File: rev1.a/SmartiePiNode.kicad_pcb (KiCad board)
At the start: 2 copper layers, 71.7 x 55 mm, 62 parts, among them CN1 USBMICROb, CN2 SWD, CN3 SX1238_TRX_HEADER, CN4 VIN, SW1 SW_PUSH, U1 ISL91127IR, U2 STM32L052_LQFP48, X1 abm10, X2 ABS25-32.768KHZ-6-T

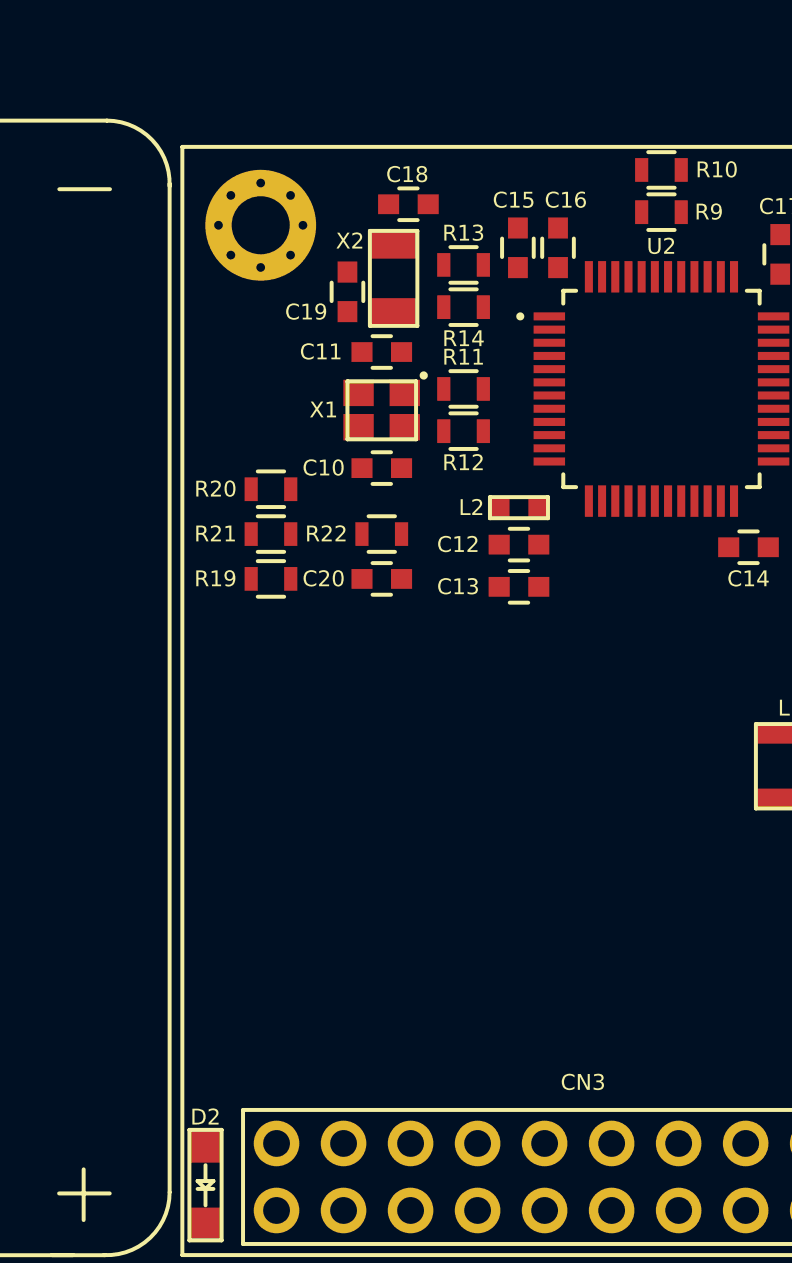
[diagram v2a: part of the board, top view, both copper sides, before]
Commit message: more layout
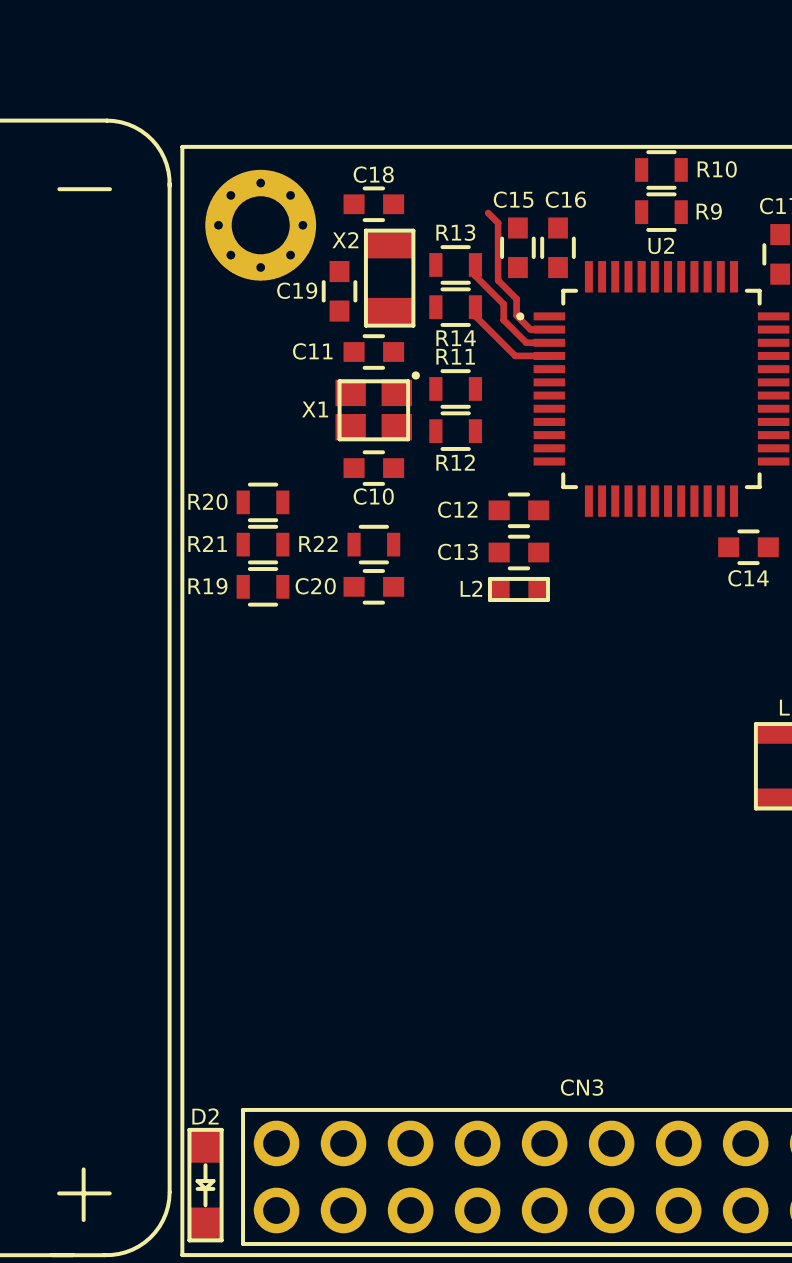
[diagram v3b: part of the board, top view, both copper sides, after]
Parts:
- moved L2 3.10 mm to (143.3, 124.8)
- moved C18 1.31 mm to (137.8, 110.2), turned to 0 degrees
- moved C12 1.30 mm to (143.3, 121.8)
- moved C13 1.30 mm to (143.3, 123.4)
- moved R20 0.58 mm to (133.6, 121.5)
- moved R21 0.50 mm to (133.6, 123.1)
- moved R22 0.50 mm to (137.8, 123.1)
- moved R19 0.42 mm to (133.6, 124.7)
- moved C20 0.42 mm to (137.8, 124.7)
- moved C19 0.30 mm to (136.5, 113.5)
- moved C10 0.30 mm to (137.8, 120.2)
- moved C11 0.30 mm to (137.8, 115.8)
- moved R11 0.30 mm to (140.9, 117.2)
- moved R12 0.30 mm to (140.9, 118.8), turned to 180 degrees
- moved R13 0.30 mm to (140.9, 112.5)
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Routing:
- net Net-(U2-Pad2): track 0.00 -> 5.80 mm
- net Net-(R13-Pad2): track 0.00 -> 4.62 mm
- net Net-(R14-Pad2): track 0.00 -> 3.77 mm
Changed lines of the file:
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@@
   (general
     (links 205)
-    (no_connects 141)
+    (no_connects 139)
     (area 98.984999 95.604999 170.825001 150.735001)
     (thickness 1.6)
     (drawings 12)
-    (tracks 1)
+    (tracks 15)
     (zones 0)
     (modules 62)
@@
   )
   (module Capacitors_SMD:C_0603 (layer F.Cu)
-    (at 138.1 120.2 180)
+    (at 137.8 120.2 180)
     (descr "Capacitor SMD 0603, reflow soldering, AVX (see smccp.pdf)")
     (tags "capacitor 0603")
     (attr smd)
-    (fp_text reference C10 (at 2.2 0 180) (layer F.SilkS)
+    (fp_text reference C10 (at 0 -1.1 180) (layer F.SilkS)
       (effects (font (size 0.6 0.6) (thickness 0.1)))
     )
@@
   )
   (module Capacitors_SMD:C_0603 (layer F.Cu)
-    (at 138.1 115.8)
+    (at 137.8 115.8)
     (descr "Capacitor SMD 0603, reflow soldering, AVX (see smccp.pdf)")
     (tags "capacitor 0603")
@@
   )
   (module Capacitors_SMD:C_0603 (layer F.Cu)
-    (at 143.3 123.1)
+    (at 143.3 121.8)
     (descr "Capacitor SMD 0603, reflow soldering, AVX (see smccp.pdf)")
     (tags "capacitor 0603")
@@
   )
   (module Capacitors_SMD:C_0603 (layer F.Cu)
-    (at 143.3 124.7)
+    (at 143.3 123.4)
     (descr "Capacitor SMD 0603, reflow soldering, AVX (see smccp.pdf)")
     (tags "capacitor 0603")
@@
   )
   (module Capacitors_SMD:C_0603 (layer F.Cu)
-    (at 139.11 110.2 180)
+    (at 137.8 110.2)
     (descr "Capacitor SMD 0603, reflow soldering, AVX (see smccp.pdf)")
     (tags "capacitor 0603")
     (attr smd)
-    (fp_text reference C18 (at 0.04 1.12 180) (layer F.SilkS)
-      (effects (font (size 0.6 0.6) (thickness 0.1)))
-    )
-    (fp_text value 4.3pF (at 0 1.9 180) (layer F.Fab)
+    (fp_text reference C18 (at 0 -1.1) (layer F.SilkS)
+      (effects (font (size 0.6 0.6) (thickness 0.1)))
+    )
+    (fp_text value 4.3pF (at 0 1.9) (layer F.Fab)
       (effects (font (size 0.6 0.6) (thickness 0.1)))
     )
@@
     (fp_line (start -1.45 0.75) (end 1.45 0.75) (layer F.CrtYd) (width 0.05))
     (fp_line (start -1.45 -0.75) (end 1.45 -0.75) (layer F.CrtYd) (width 0.05))
-    (pad 2 smd rect (at 0.75 0 180) (size 0.8 0.75) (layers F.Cu F.Paste F.Mask)
+    (pad 2 smd rect (at 0.75 0) (size 0.8 0.75) (layers F.Cu F.Paste F.Mask)
       (net 10 "Net-(C18-Pad2)"))
-    (pad 1 smd rect (at -0.75 0 180) (size 0.8 0.75) (layers F.Cu F.Paste F.Mask)
+    (pad 1 smd rect (at -0.75 0) (size 0.8 0.75) (layers F.Cu F.Paste F.Mask)
       (net 1 GND))
     (model Capacitors_SMD.3dshapes/C_0603.wrl
@@
   )
   (module Capacitors_SMD:C_0603 (layer F.Cu)
-    (at 136.8 113.52 270)
+    (at 136.5 113.5 270)
     (descr "Capacitor SMD 0603, reflow soldering, AVX (see smccp.pdf)")
     (tags "capacitor 0603")
     (attr smd)
-    (fp_text reference C19 (at 0.77 1.56) (layer F.SilkS)
+    (fp_text reference C19 (at 0 1.6) (layer F.SilkS)
       (effects (font (size 0.6 0.6) (thickness 0.1)))
     )
@@
   )
   (module Resistors_SMD:R_0603 (layer F.Cu)
-    (at 141.2 117.2 180)
+    (at 140.9 117.2 180)
     (descr "Resistor SMD 0603, reflow soldering, Vishay (see dcrcw.pdf)")
     (tags "resistor 0603")
@@
   )
   (module Resistors_SMD:R_0603 (layer F.Cu)
-    (at 141.2 118.8)
+    (at 140.9 118.8 180)
     (descr "Resistor SMD 0603, reflow soldering, Vishay (see dcrcw.pdf)")
     (tags "resistor 0603")
     (attr smd)
-    (fp_text reference R12 (at 0 1.2) (layer F.SilkS)
-      (effects (font (size 0.6 0.6) (thickness 0.1)))
-    )
-    (fp_text value DNP (at 0 1.9) (layer F.Fab)
+    (fp_text reference R12 (at 0 -1.22 180) (layer F.SilkS)
+      (effects (font (size 0.6 0.6) (thickness 0.1)))
+    )
+    (fp_text value DNP (at 0 1.9 180) (layer F.Fab)
       (effects (font (size 0.6 0.6) (thickness 0.1)))
     )
@@
     (fp_line (start -1.3 0.8) (end 1.3 0.8) (layer F.CrtYd) (width 0.05))
     (fp_line (start -1.3 -0.8) (end 1.3 -0.8) (layer F.CrtYd) (width 0.05))
-    (pad 2 smd rect (at 0.75 0) (size 0.5 0.9) (layers F.Cu F.Paste F.Mask)
+    (pad 2 smd rect (at 0.75 0 180) (size 0.5 0.9) (layers F.Cu F.Paste F.Mask)
       (net 7 "Net-(C10-Pad2)"))
-    (pad 1 smd rect (at -0.75 0) (size 0.5 0.9) (layers F.Cu F.Paste F.Mask)
+    (pad 1 smd rect (at -0.75 0 180) (size 0.5 0.9) (layers F.Cu F.Paste F.Mask)
       (net 41 "Net-(R12-Pad1)"))
     (model Resistors_SMD.3dshapes/R_0603.wrl
@@
   )
   (module Resistors_SMD:R_0603 (layer F.Cu)
-    (at 141.2 112.5)
+    (at 140.9 112.5)
     (descr "Resistor SMD 0603, reflow soldering, Vishay (see dcrcw.pdf)")
     (tags "resistor 0603")
@@
   )
   (module Resistors_SMD:R_0603 (layer F.Cu)
-    (at 141.2 114.1)
+    (at 140.9 114.1)
     (descr "Resistor SMD 0603, reflow soldering, Vishay (see dcrcw.pdf)")
     (tags "resistor 0603")
@@
   )
   (module abracon-abm10:abracon-abm10 (layer F.Cu)
-    (at 138.1 118 180)
+    (at 137.8 118 180)
     (fp_text reference X1 (at 2.2 0 180) (layer F.SilkS)
       (effects (font (size 0.6 0.6) (thickness 0.1)))
@@
     (descr "Through hole pin header")
     (tags "pin header")
-    (fp_text reference CN3 (at -2.31 11.24) (layer F.SilkS)
+    (fp_text reference CN3 (at -2.096 11.272) (layer F.SilkS)
       (effects (font (size 0.6 0.6) (thickness 0.1)))
     )
@@
   )
   (module abracon-abs07:abracon-abs07 (layer F.Cu)
-    (at 138.55 113.01 90)
+    (at 138.4 113 90)
     (fp_text reference X2 (at 1.41 -1.65 180) (layer F.SilkS)
       (effects (font (size 0.6 0.6) (thickness 0.1)))
@@
   )
   (module bourns-MH1608-601Y:MH1608-601Y (layer F.Cu)
-    (at 143.3 121.7)
+    (at 143.3 124.8)
     (fp_text reference L2 (at -1.8 0) (layer F.SilkS)
       (effects (font (size 0.6 0.6) (thickness 0.1)))
@@
   )
   (module Capacitors_SMD:C_0603 (layer F.Cu)
-    (at 138.1 124.4 180)
+    (at 137.8 124.7 180)
     (descr "Capacitor SMD 0603, reflow soldering, AVX (see smccp.pdf)")
     (tags "capacitor 0603")
@@
   )
   (module Resistors_SMD:R_0603 (layer F.Cu)
-    (at 133.9 124.4)
+    (at 133.6 124.7)
     (descr "Resistor SMD 0603, reflow soldering, Vishay (see dcrcw.pdf)")
     (tags "resistor 0603")
@@
   )
   (module Resistors_SMD:R_0603 (layer F.Cu)
-    (at 133.9 121 180)
+    (at 133.6 121.5 180)
     (descr "Resistor SMD 0603, reflow soldering, Vishay (see dcrcw.pdf)")
     (tags "resistor 0603")
@@
   )
   (module Resistors_SMD:R_0603 (layer F.Cu)
-    (at 133.9 122.7)
+    (at 133.6 123.1)
     (descr "Resistor SMD 0603, reflow soldering, Vishay (see dcrcw.pdf)")
     (tags "resistor 0603")
@@
   )
   (module Resistors_SMD:R_0603 (layer F.Cu)
-    (at 138.1 122.7 180)
+    (at 137.8 123.1 180)
     (descr "Resistor SMD 0603, reflow soldering, Vishay (see dcrcw.pdf)")
     (tags "resistor 0603")
@@
   (gr_arc (start 100.64 149.08) (end 100.64 150.66) (angle 90) (layer Edge.Cuts) (width 0.15))
   (segment (start 157.03 140.83) (end 157.03 140.46) (width 0.25) (layer F.Cu) (net 3))
+  (segment (start 142.72 113.99) (end 141.65 112.92) (width 0.25) (layer F.Cu) (net 42))
+  (segment (start 141.65 112.92) (end 141.65 112.5) (width 0.25) (layer F.Cu) (net 42))
+  (segment (start 142.72 114.59) (end 142.72 113.99) (width 0.25) (layer F.Cu) (net 42))
+  (segment (start 143.580001 115.450001) (end 142.72 114.59) (width 0.25) (layer F.Cu) (net 42))
+  (segment (start 144.450001 115.450001) (end 143.580001 115.450001) (width 0.25) (layer F.Cu) (net 42))
+  (segment (start 143.16 115.95) (end 141.65 114.44) (width 0.25) (layer F.Cu) (net 43))
+  (segment (start 141.65 114.44) (end 141.65 114.1) (width 0.25) (layer F.Cu) (net 43))
+  (segment (start 144.450001 115.95) (end 143.16 115.95) (width 0.25) (layer F.Cu) (net 43))
+  (segment (start 142.51 110.91) (end 142.13 110.53) (width 0.25) (layer F.Cu) (net 71))
+  (segment (start 142.51 113.09) (end 142.51 110.91) (width 0.25) (layer F.Cu) (net 71))
+  (segment (start 143.21 113.79) (end 142.51 113.09) (width 0.25) (layer F.Cu) (net 71))
+  (segment (start 143.21 114.42) (end 143.21 113.79) (width 0.25) (layer F.Cu) (net 71))
+  (segment (start 143.739999 114.949999) (end 143.21 114.42) (width 0.25) (layer F.Cu) (net 71))
+  (segment (start 144.450001 114.949999) (end 143.739999 114.949999) (width 0.25) (layer F.Cu) (net 71))
 )

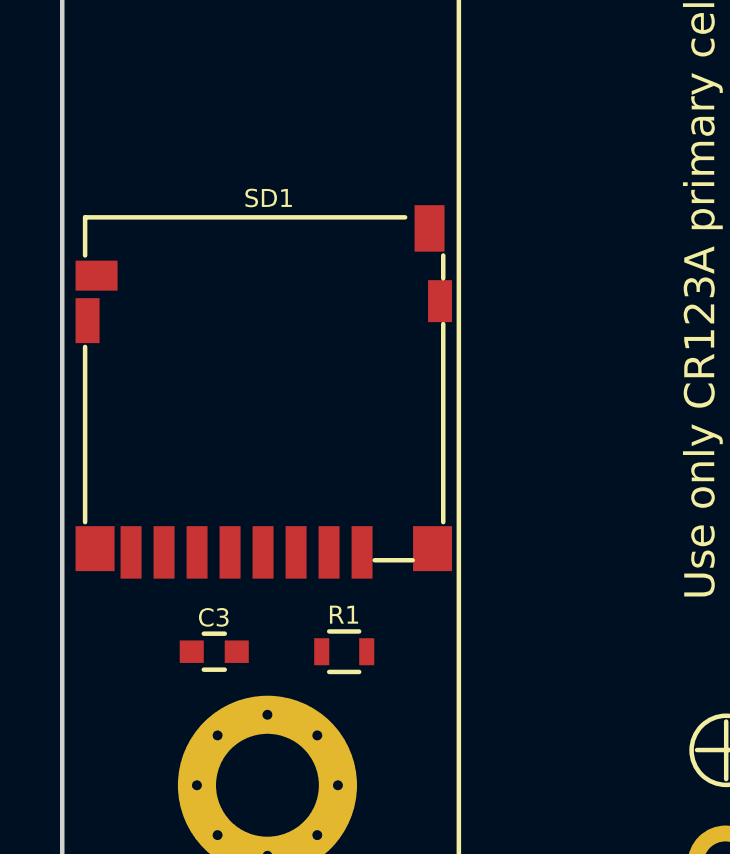
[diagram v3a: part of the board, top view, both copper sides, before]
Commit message: optimizing nets
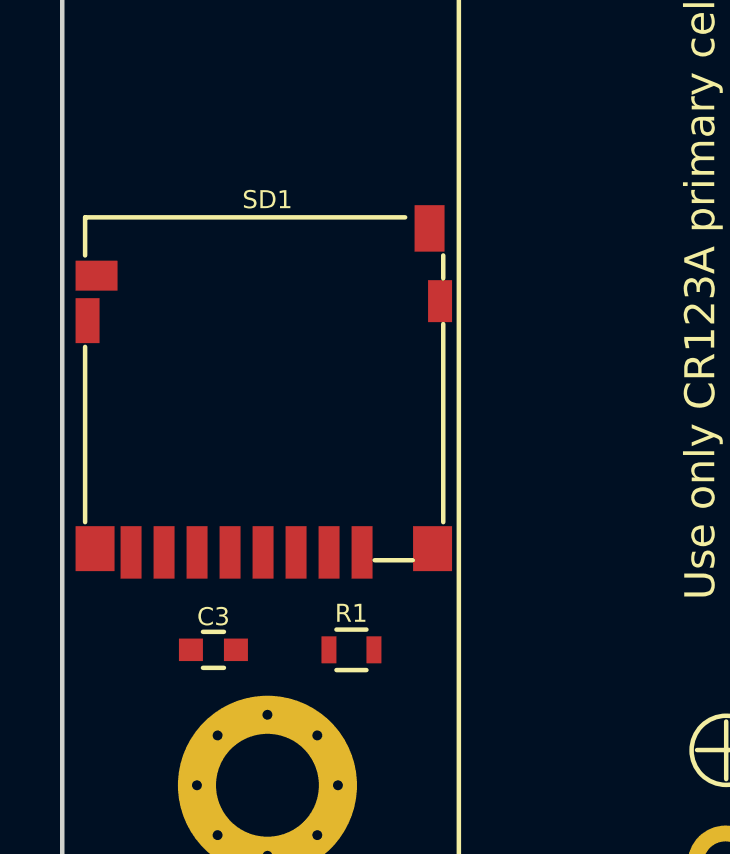
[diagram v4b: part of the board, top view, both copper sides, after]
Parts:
- moved R1 0.25 mm to (108.7, 140.4)
- moved C3 0.07 mm to (104.1, 140.4), turned to 180 degrees
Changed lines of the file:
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@@
   )
   (module Capacitors_SMD:C_0603 (layer F.Cu)
-    (at 104.128 140.462)
-    (descr "Capacitor SMD 0603, reflow soldering, AVX (see smccp.pdf)")
-    (tags "capacitor 0603")
-    (attr smd)
-    (fp_text reference C3 (at -0.008 -1.122) (layer F.SilkS)
-      (effects (font (size 0.6 0.6) (thickness 0.1)))
-    )
-    (fp_text value .1uF (at 0 1.9) (layer F.Fab)
-      (effects (font (size 0.6 0.6) (thickness 0.1)))
-    )
-    (fp_line (start 0.35 0.6) (end -0.35 0.6) (layer F.SilkS) (width 0.15))
-    (fp_line (start -0.35 -0.6) (end 0.35 -0.6) (layer F.SilkS) (width 0.15))
-    (fp_line (start 1.45 -0.75) (end 1.45 0.75) (layer F.CrtYd) (width 0.05))
-    (fp_line (start -1.45 -0.75) (end -1.45 0.75) (layer F.CrtYd) (width 0.05))
-    (fp_line (start -1.45 0.75) (end 1.45 0.75) (layer F.CrtYd) (width 0.05))
-    (fp_line (start -1.45 -0.75) (end 1.45 -0.75) (layer F.CrtYd) (width 0.05))
-    (pad 2 smd rect (at 0.75 0) (size 0.8 0.75) (layers F.Cu F.Paste F.Mask)
-      (net 1 GND))
-    (pad 1 smd rect (at -0.75 0) (size 0.8 0.75) (layers F.Cu F.Paste F.Mask)
+    (at 104.1 140.4 180)
+    (descr "Capacitor SMD 0603, reflow soldering, AVX (see smccp.pdf)")
+    (tags "capacitor 0603")
+    (attr smd)
+    (fp_text reference C3 (at 0 1.1 180) (layer F.SilkS)
+      (effects (font (size 0.6 0.6) (thickness 0.1)))
+    )
+    (fp_text value .1uF (at 0 1.9 180) (layer F.Fab)
+      (effects (font (size 0.6 0.6) (thickness 0.1)))
+    )
+    (fp_line (start 0.35 0.6) (end -0.35 0.6) (layer F.SilkS) (width 0.15))
+    (fp_line (start -0.35 -0.6) (end 0.35 -0.6) (layer F.SilkS) (width 0.15))
+    (fp_line (start 1.45 -0.75) (end 1.45 0.75) (layer F.CrtYd) (width 0.05))
+    (fp_line (start -1.45 -0.75) (end -1.45 0.75) (layer F.CrtYd) (width 0.05))
+    (fp_line (start -1.45 0.75) (end 1.45 0.75) (layer F.CrtYd) (width 0.05))
+    (fp_line (start -1.45 -0.75) (end 1.45 -0.75) (layer F.CrtYd) (width 0.05))
+    (pad 2 smd rect (at 0.75 0 180) (size 0.8 0.75) (layers F.Cu F.Paste F.Mask)
+      (net 1 GND))
+    (pad 1 smd rect (at -0.75 0 180) (size 0.8 0.75) (layers F.Cu F.Paste F.Mask)
       (net 4 /+3V3))
     (model Capacitors_SMD.3dshapes/C_0603.wrl
@@
   )
   (module Resistors_SMD:R_0603 (layer F.Cu)
-    (at 108.458 140.462 180)
+    (at 108.7 140.4 180)
     (descr "Resistor SMD 0603, reflow soldering, Vishay (see dcrcw.pdf)")
     (tags "resistor 0603")
@@
   (module amphenol-microsd-114-00841-68:amphenol-microsd-1140084168 (layer F.Cu)
     (at 105.918 131.572)
-    (fp_text reference SD1 (at 0.032 -6.212) (layer F.SilkS)
-      (effects (font (size 0.6 0.6) (thickness 0.1)))
-    )
+    (fp_text reference SD1 (at -0.018 -6.172) (layer F.SilkS)
+      (effects (font (size 0.6 0.6) (thickness 0.1)))
+    )
